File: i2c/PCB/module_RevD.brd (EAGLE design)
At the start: 33.3 x 50.2 mm, 131 parts, among them IC1 ATTINY85-20SU, J1 M20-9980346

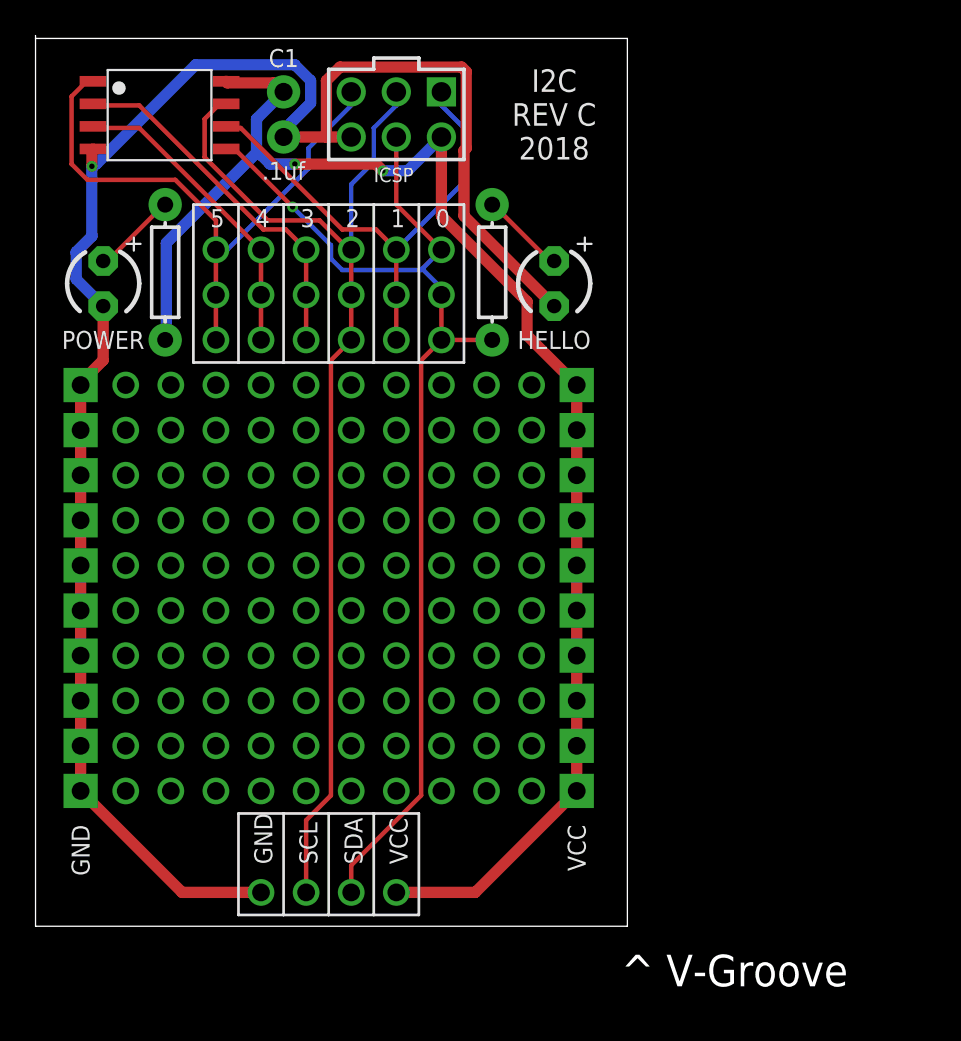
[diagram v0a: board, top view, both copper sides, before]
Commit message: Rework of revD boards
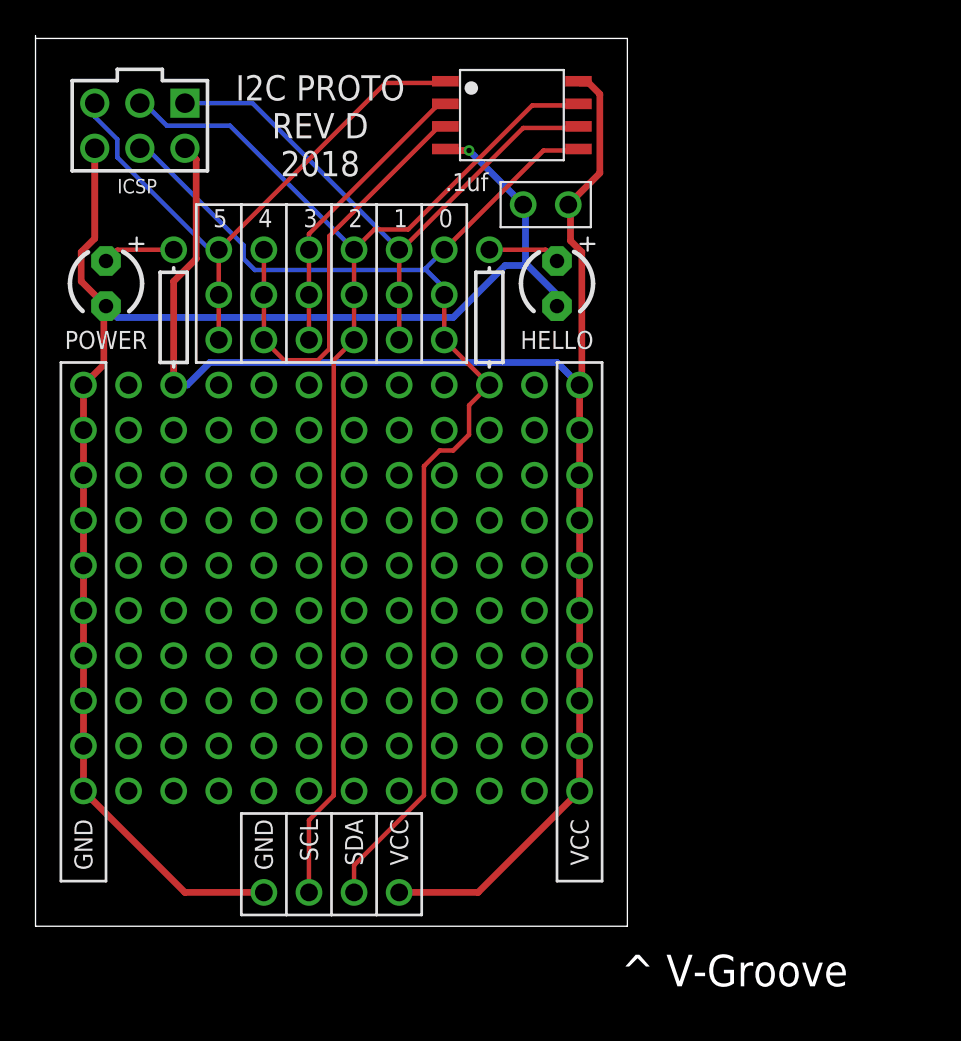
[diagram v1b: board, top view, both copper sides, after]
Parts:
- removed GND, VCC: 10X-PADS, BadgeParts:10X-PADS
- removed R1, R2: 220, SparkFun-Resistors:AXIAL-0.3
- added U$124, U$125, U$128, U$129, U$130, U$131, U$132, U$133, U$134, U$135, U$136, U$137, U$138, U$139, U$140, U$141, U$142, U$143: ONE_PAD, BadgeParts:1X01
- added U$126, U$127: RESISTOR, BadgeParts:AXIAL-0.3
- moved U$100 22.7 mm to (2.70, 30.5), turned to 0 degrees
- moved IC1 19.8 mm to (26.8, 45.7)
- moved J1 14.5 mm to (5.88, 42.5)
- moved U$123 14.0 mm to (27.5, 40.6), turned to 0 degrees
- moved U$99 13.6 mm to (2.70, 17.8), turned to 0 degrees
- moved HELLO 0.16 mm to (29.4, 36.2)
- moved POWER 0.16 mm to (3.97, 36.2)
- moved U$1 0.16 mm to (7.78, 15.2)
- moved U$10 0.16 mm to (7.78, 12.7)
- moved U$101 0.16 mm to (10.3, 25.4)
- moved U$102 0.16 mm to (10.3, 27.9)
- moved U$103 0.16 mm to (10.3, 30.5)
- moved U$104 0.16 mm to (28.1, 30.5)
- moved U$105 0.16 mm to (12.9, 25.4)
- moved U$106 0.16 mm to (12.9, 27.9)
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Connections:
- removed net N$3: HELLO.POS, R2.P$1
- new net N$2: HELLO.POS, U$127.P$3
- net GND: now also U$100.P$1, U$123.P$1, U$124.P$1, U$125.P$1, U$128.P$1, U$129.P$1, U$130.P$1, U$131.P$1, U$132.P$1, U$133.P$1, U$99.P$1; no longer GND.P$1, GND.P$10, GND.P$2, GND.P$3, GND.P$4, GND.P$5, GND.P$6, GND.P$7, GND.P$8, GND.P$9, U$123.1
- net N$1: now also U$126.P$3; no longer R1.P$1
- net PB0: now also U$127.P$4; no longer R2.P$2
- net VCC: now also U$123.P$2, U$126.P$4, U$134.P$1, U$135.P$1, U$136.P$1, U$137.P$1, U$138.P$1, U$139.P$1, U$140.P$1, U$141.P$1, U$142.P$1, U$143.P$1; no longer R1.P$2, U$123.2, VCC.P$1, VCC.P$10, VCC.P$2, VCC.P$3, VCC.P$4, VCC.P$5, VCC.P$6, VCC.P$7, VCC.P$8, VCC.P$9
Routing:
- net GND: track 99.7 -> 87.5 mm
- net VCC: track 84.4 -> 92.4 mm, vias 2 -> 0
- net PB4: track 17.4 -> 25.0 mm
- net PB2: track 61.3 -> 68.8 mm
- net PB0: track 63.8 -> 71.0 mm, vias 1 -> 0
- net PB1: track 28.5 -> 33.5 mm
- net N$3: track 4.81 -> 0.00 mm
- net N$2: track 0.00 -> 4.07 mm
- net PB3: track 20.5 -> 16.7 mm
- net PB5: track 34.0 -> 33.2 mm
- net N$1: track 4.81 -> 4.07 mm
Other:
- board text added: "I2C PROTO REV D 2018"
- board text removed: "C1"
- board text removed: "I2C REV C 2018"
